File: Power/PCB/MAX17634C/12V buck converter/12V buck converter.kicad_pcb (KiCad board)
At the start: 4 copper layers, 24.5 x 24.5 mm, 10 parts

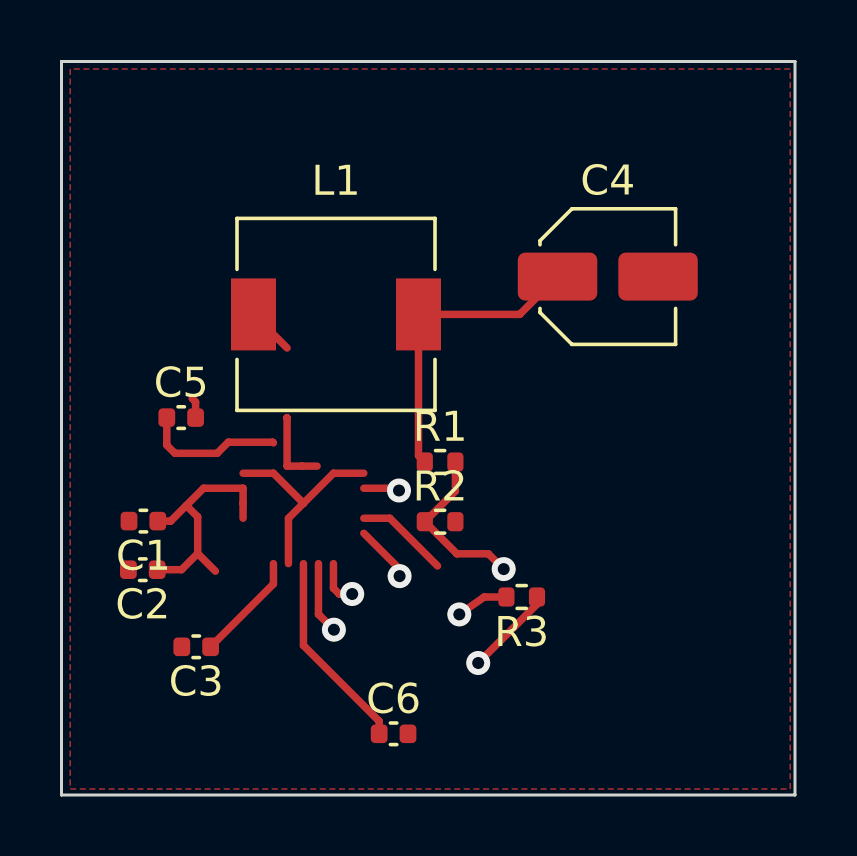
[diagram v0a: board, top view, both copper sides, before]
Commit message: PS drawio IC update
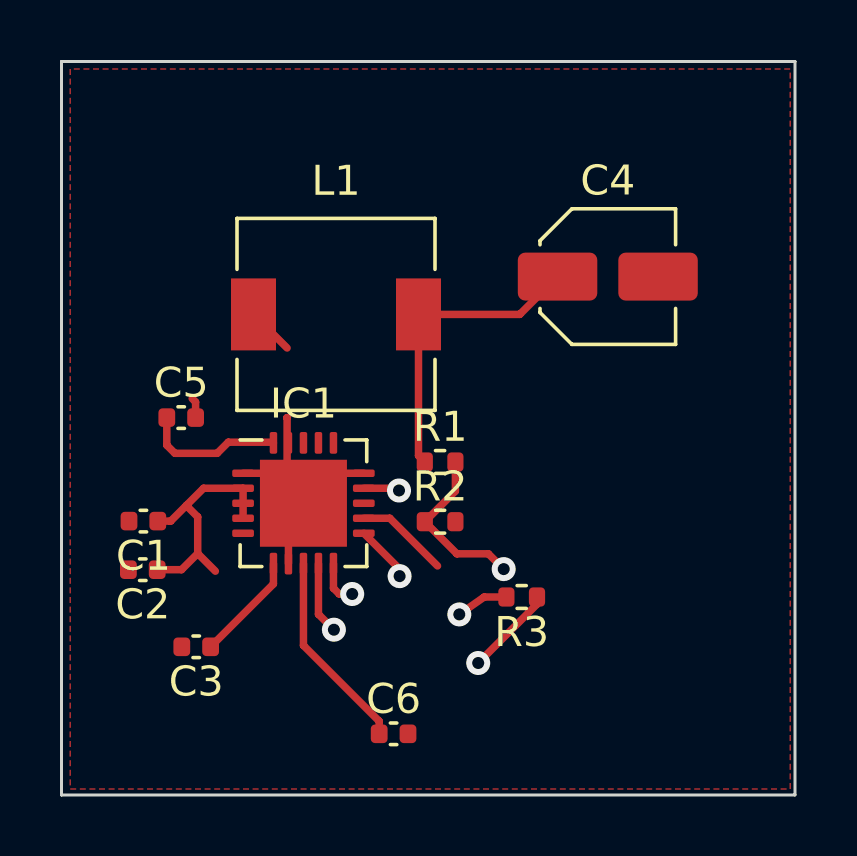
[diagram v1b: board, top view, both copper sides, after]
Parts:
- added IC1: MAX17634C, Package_DFN_QFN:TQFN-20-1EP_4x4mm_P0.5mm_EP2.9x2.9mm, F.Cu at (111.8, 66.0)
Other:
- copper layers 4 -> 32
